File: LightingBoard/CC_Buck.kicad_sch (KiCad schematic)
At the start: 18 parts, among them J8 LED Out, U11 TPS62933FDRLR, U12 MCP6486

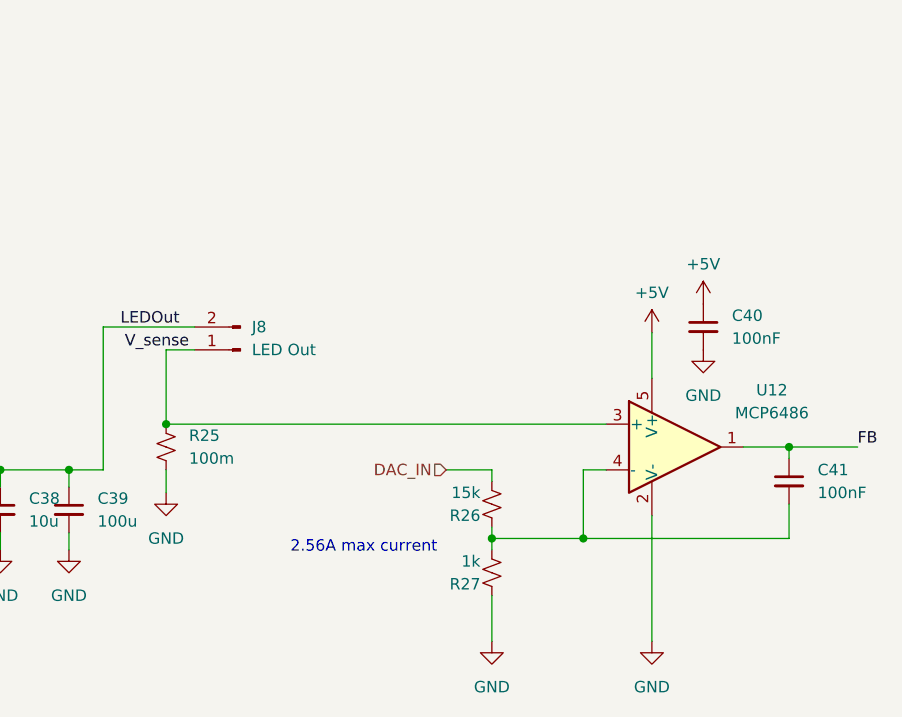
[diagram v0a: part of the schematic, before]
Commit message: fabbed
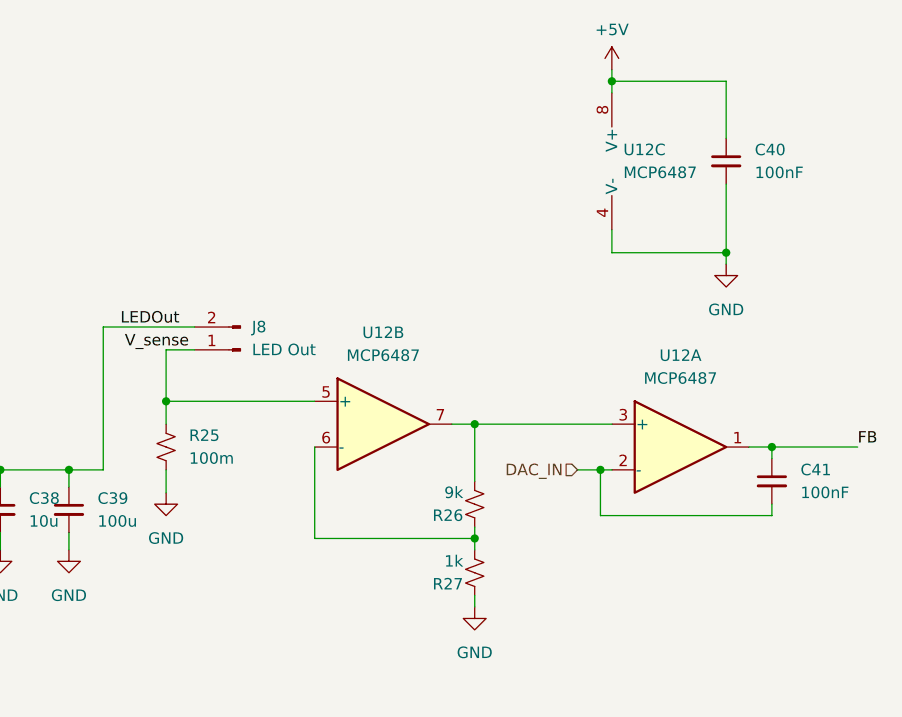
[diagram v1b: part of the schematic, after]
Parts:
- removed U12: MCP6486, Package_TO_SOT_SMD:SOT-353_SC-70-5, symbol CustomSymbols:TL081HIDCKR
- added U12: MCP6487, Package_SO:MSOP-8_3x3mm_P0.65mm, symbol Amplifier_Operational:TLV2372
- R26: value 15k -> 9k
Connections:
- net +5V: now also U12.8 (V+)
- net DAC_IN: now also C41.2, U12.2 (-); no longer R26.1
- net FB: now also U12.1
- net GND: now also U12.4 (V-)
- net V_sense: now also U12.5 (+)
- net at R26.2, R27.1: now also U12.6 (-); no longer C41.2
- new net: R26.1, U12.3 (+), U12.7
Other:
- note removed: "2.56A max current"
- moved on the sheet: C40, C41, R26, R27
